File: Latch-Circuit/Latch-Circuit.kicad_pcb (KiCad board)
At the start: 2 copper layers, 90 x 50 mm, 96 parts, among them J1 BM02B-PASS-1-TF, J10 BM02B-PASS-1-TF, J2 BM03B-PASS-1-TF, J3 BM02B-PASS-1-TF, J4 BM02B-PASS-1-TF, J5 BM02B-PASS-1-TF, J6 BM02B-PASS-1-TF, J7 B2P-VH, J8 BM02B-PASS-1-TF, J9 BM02B-PASS-1-TF, K1 G5Q-1A4_DC12, K2 G5Q-1A4_DC12, K3 G5Q-1A4_DC12, Q1 DMP3098LQ-7, Q10 2N7002K-AU, Q11 2N7002K-AU, Q12 PJA3439-AU_R1_000A1, Q13 PJA3439-AU_R1_000A1, Q2 2N7002K-AU, Q3 PJA3439-AU_R1_000A1, Q4 2N7002K-AU, Q5 PJA3439-AU_R1_000A1, Q6 2N7002K-AU, Q7 2N7002K-AU, Q8 PJA3439-AU_R1_000A1, Q9 PJA3439-AU_R1_000A1

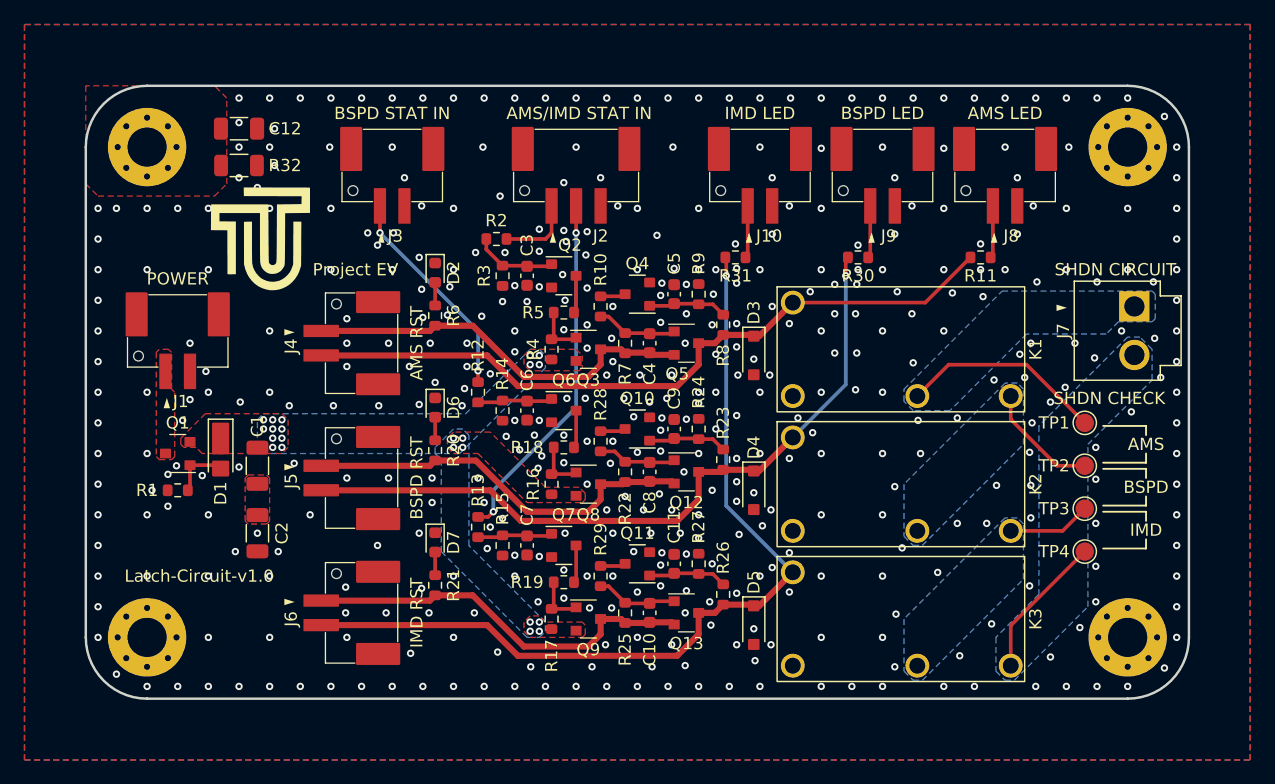
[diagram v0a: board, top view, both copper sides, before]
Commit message: 配置、配線終了
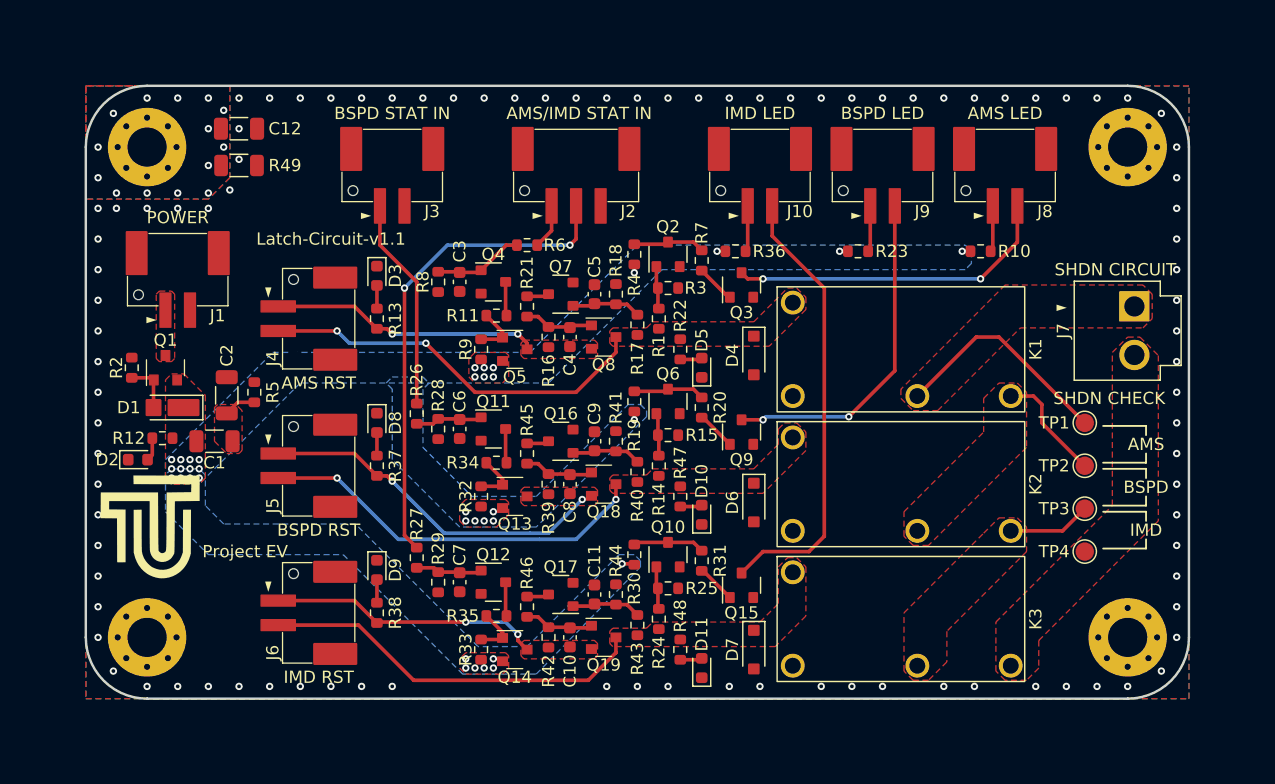
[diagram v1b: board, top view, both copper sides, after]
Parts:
- added D10: LED, LED_SMD:LED_0603_1608Metric, F.Cu at (50.2, 35.0)
- added D11: LED, LED_SMD:LED_0603_1608Metric, F.Cu at (50.2, 47.5)
- added D2: LED, LED_SMD:LED_0603_1608Metric, F.Cu at (4.25, 30.5)
- added D5: LED, LED_SMD:LED_0603_1608Metric, F.Cu at (50.2, 23.0)
- added Q10: 2N7002K-AU, ProjectEV:Package_SOT-23_2N7002K-AU, F.Cu at (47.5, 38.2)
- added Q15: 2N7002K-AU, ProjectEV:Package_SOT-23_2N7002K-AU, F.Cu at (53.5, 40.8)
- added Q2: 2N7002K-AU, ProjectEV:Package_SOT-23_2N7002K-AU, F.Cu at (47.5, 13.8)
- added Q3: 2N7002K-AU, ProjectEV:Package_SOT-23_2N7002K-AU, F.Cu at (53.5, 16.2)
- added Q6: 2N7002K-AU, ProjectEV:Package_SOT-23_2N7002K-AU, F.Cu at (47.5, 25.8)
- added Q9: 2N7002K-AU, ProjectEV:Package_SOT-23_2N7002K-AU, F.Cu at (53.5, 28.2)
- added R1: 100, Resistor_SMD:R_0603_1608Metric, F.Cu at (46.8, 19.0)
- added R12: 10k, Resistor_SMD:R_0603_1608Metric, F.Cu at (6.25, 28.8)
- added R14: 100, Resistor_SMD:R_0603_1608Metric, F.Cu at (46.8, 31.0)
- added R15: 100k, Resistor_SMD:R_0603_1608Metric, F.Cu at (47.5, 28.5)
- added R19: 100k, Resistor_SMD:R_0603_1608Metric, F.Cu at (44.8, 25.8)
- added R20: 100, Resistor_SMD:R_0603_1608Metric, F.Cu at (50.2, 26.2)
- added R22: 10k, Resistor_SMD:R_0603_1608Metric, F.Cu at (48.5, 21.5)
- added R24: 100, Resistor_SMD:R_0603_1608Metric, F.Cu at (46.8, 43.5)
- added R25: 100k, Resistor_SMD:R_0603_1608Metric, F.Cu at (47.5, 41.0)
- added R3: 100k, Resistor_SMD:R_0603_1608Metric, F.Cu at (47.5, 16.5)
- added R30: 100k, Resistor_SMD:R_0603_1608Metric, F.Cu at (44.8, 38.2)
- added R31: 100, Resistor_SMD:R_0603_1608Metric, F.Cu at (50.2, 38.8)
- added R4: 100k, Resistor_SMD:R_0603_1608Metric, F.Cu at (44.8, 13.8)
- added R47: 10k, Resistor_SMD:R_0603_1608Metric, F.Cu at (48.5, 33.5)
- added R48: 10k, Resistor_SMD:R_0603_1608Metric, F.Cu at (48.5, 46.0)
- added R5: 1M, Resistor_SMD:R_0603_1608Metric, F.Cu at (13.8, 25.0)
- added R7: 100, Resistor_SMD:R_0603_1608Metric, F.Cu at (50.2, 14.2)
- R16: renamed from R7; value 1M -> 100k
- R18: renamed from R9; value 1M -> 100k
- R28: renamed from R14; value 1M -> 100k
- R29: renamed from R15; value 1M -> 100k
- R32: renamed from R16; value 1M -> 100k
- R33: renamed from R17; value 1M -> 100k
- R39: renamed from R22; value 1M -> 100k
- R41: renamed from R24; value 1M -> 100k
- R42: renamed from R25; value 1M -> 100k
- R44: renamed from R27; value 1M -> 100k
- R8: renamed from R3; value 1M -> 100k
- R9: renamed from R4; value 1M -> 100k
- moved G*** 25.2 mm to (5.00, 36.0)
- moved C2 11.5 mm to (11.5, 25.2), turned to 90 degrees
- moved R2 10.7 mm to (3.75, 23.0), turned to -90 degrees
- moved R43 7.43 mm to (45.0, 44.0)
- moved R44 7.20 mm to (43.2, 41.5)
- moved Q1 7.07 mm to (6.50, 23.0), turned to 0 degrees
- moved R40 7.07 mm to (45.0, 31.5)
- moved Q19 7.04 mm to (42.2, 45.0)
- moved R17 7.00 mm to (45.0, 19.5)
- moved C11 6.96 mm to (41.5, 41.5)
- moved Q18 6.82 mm to (42.2, 32.5)
- moved R41 6.82 mm to (43.2, 29.0)
- moved C10 6.80 mm to (39.5, 45.0)
- moved Q8 6.77 mm to (42.2, 20.5)
- moved R18 6.75 mm to (43.2, 17.0)
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- renumbered D2 to D3, D3 to D4, D4 to D6, D5 to D7, D6 to D8, D7 to D9, Q6 to Q11, Q7 to Q12, Q8 to Q13, Q9 to Q14, Q10 to Q16, Q11 to Q17, Q12 to Q18, Q13 to Q19, Q2 to Q4, Q3 to Q5, Q4 to Q7, Q5 to Q8, R11 to R10, R5 to R11, R6 to R13, R8 to R17, R1 to R2, R10 to R21, R30 to R23, R12 to R26, R13 to R27, R18 to R34, R19 to R35, R31 to R36, R20 to R37, R21 to R38, R23 to R40, R26 to R43, R28 to R45, R29 to R46, R32 to R49, R2 to R6
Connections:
- J10 pad 2: GND -> /IMD_LED_K
- J8 pad 2: GND -> /AMS_LED_K
- J9 pad 2: GND -> /BSPD_LED_K
- R10 pad 2: /AMS_RELAY_DRIVE -> +12V
- R23 pad 2: /BSPD_RELAY_DRIVE -> +12V
- R36 pad 2: /IMD_RELAY_DRIVE -> +12V
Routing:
- net /IMD_RELAY_DRIVE: track 71.4 -> 31.6 mm, vias 1 -> 0
- net /IMD_LED_K: track 0.00 -> 36.7 mm
- net /BSPD_RELAY_DRIVE: track 60.3 -> 32.2 mm, vias 1 -> 2
- net /BSPD_LED_K: track 0.00 -> 27.6 mm, vias 0 -> 2
- net /AMS_RELAY_DRIVE: track 59.5 -> 32.2 mm, vias 0 -> 2
- net /AMS_LED_K: track 0.00 -> 26.9 mm, vias 0 -> 2
- net /SHDN_OUT: track 11.8 -> 0.00 mm
- net /IMD_STATUS: track 29.2 -> 39.9 mm
- net /TO_AMS_RST_SW: track 32.6 -> 22.0 mm, vias 0 -> 2
- net /TO_IMD_RST_SW: track 32.6 -> 22.3 mm, vias 0 -> 2
- net Net-(Q6-D): track 0.00 -> 5.85 mm
- net Net-(Q2-D): track 0.00 -> 5.85 mm
- net Net-(Q10-D): track 0.00 -> 5.85 mm
- net +12V: track 0.00 -> 4.41 mm, vias 22 -> 36
- net /TO_BSPD_RST_SW: track 32.5 -> 28.6 mm, vias 0 -> 2
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- added copper zone on F.Cu, net /AMS_RELAY_DRIVE
- added copper zone on F.Cu, net /BSPD_RELAY_DRIVE
- added copper zone on F.Cu, net /IMD_RELAY_DRIVE
- added copper zone on F.Cu, net /SHDN_IN
- added copper zone on F.Cu, net /SHDN_OUT
- added copper zone on F.Cu, net /TO_AMS_RST_SW
- added copper zone on F.Cu, net /TO_BSPD_RST_SW
- added copper zone on F.Cu, net /TO_IMD_RST_SW
- added copper zone on B.Cu, net Net-(C12-Pad1)
- added copper zone on F.Cu, net Net-(K1-Pad3)
- added copper zone on F.Cu, net Net-(K2-Pad3)
- removed copper zone on B.Cu, net /SHDN_IN
- removed copper zone on B.Cu, net /SHDN_OUT
- removed copper zone on B.Cu, net Net-(K1-Pad3)
- removed copper zone on B.Cu, net Net-(K2-Pad3)
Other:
- board text added: "Latch-Circuit-v1.1"
- board text removed: "Latch-Circuit-v1.0"

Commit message: complete AW, DRC next->select parts at JLCPCB
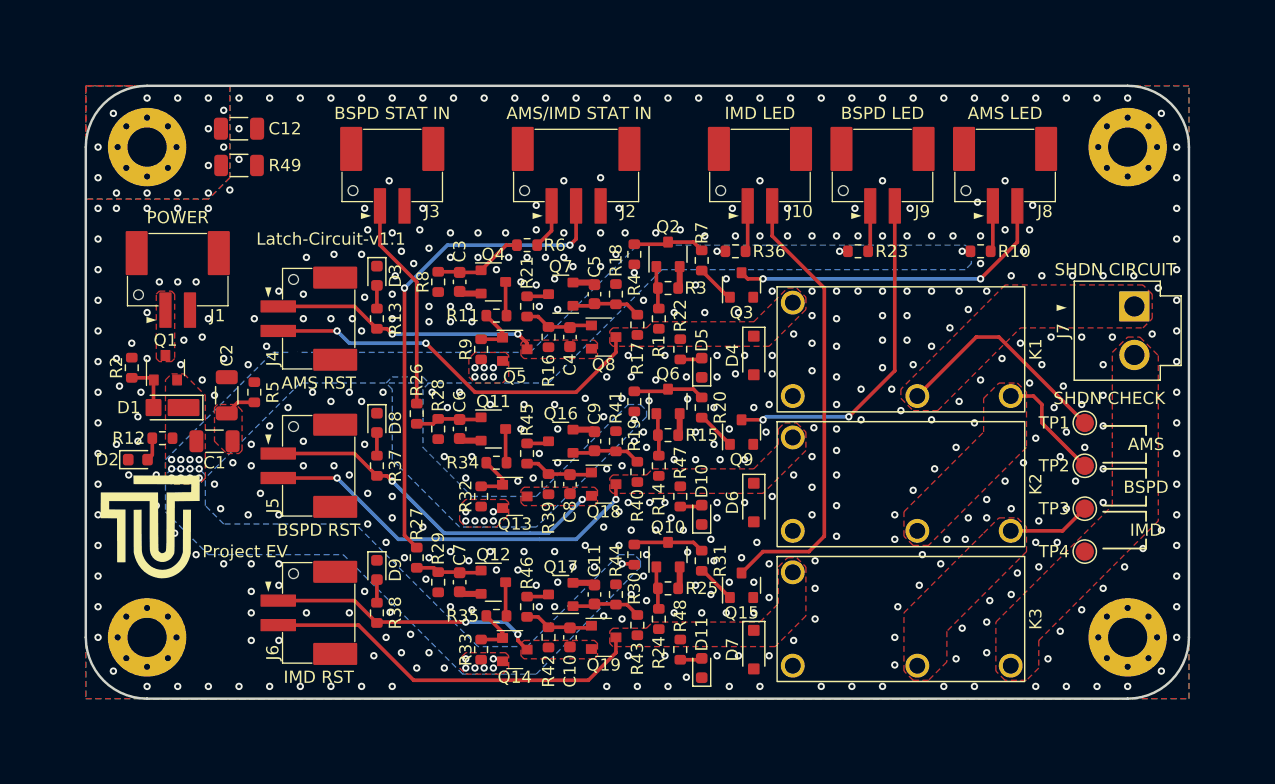
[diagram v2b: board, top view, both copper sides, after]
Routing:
- net GND: track 0.00 -> 16.3 mm, vias 95 -> 476
